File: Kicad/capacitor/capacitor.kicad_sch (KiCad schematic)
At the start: 141 parts, among them K1 Capacitor

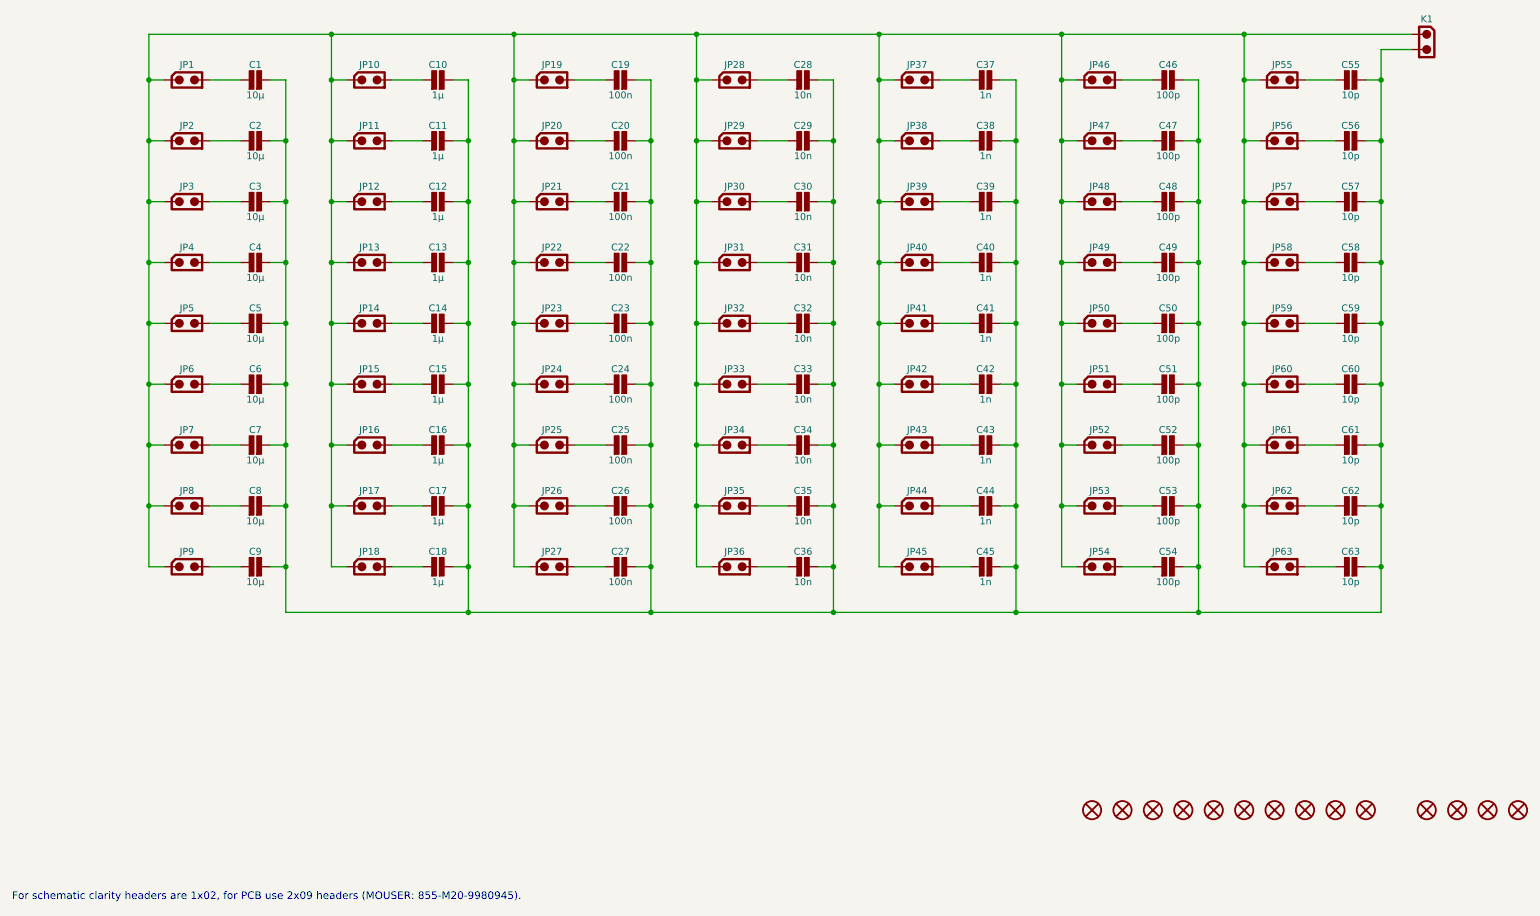
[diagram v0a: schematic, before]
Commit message: Up
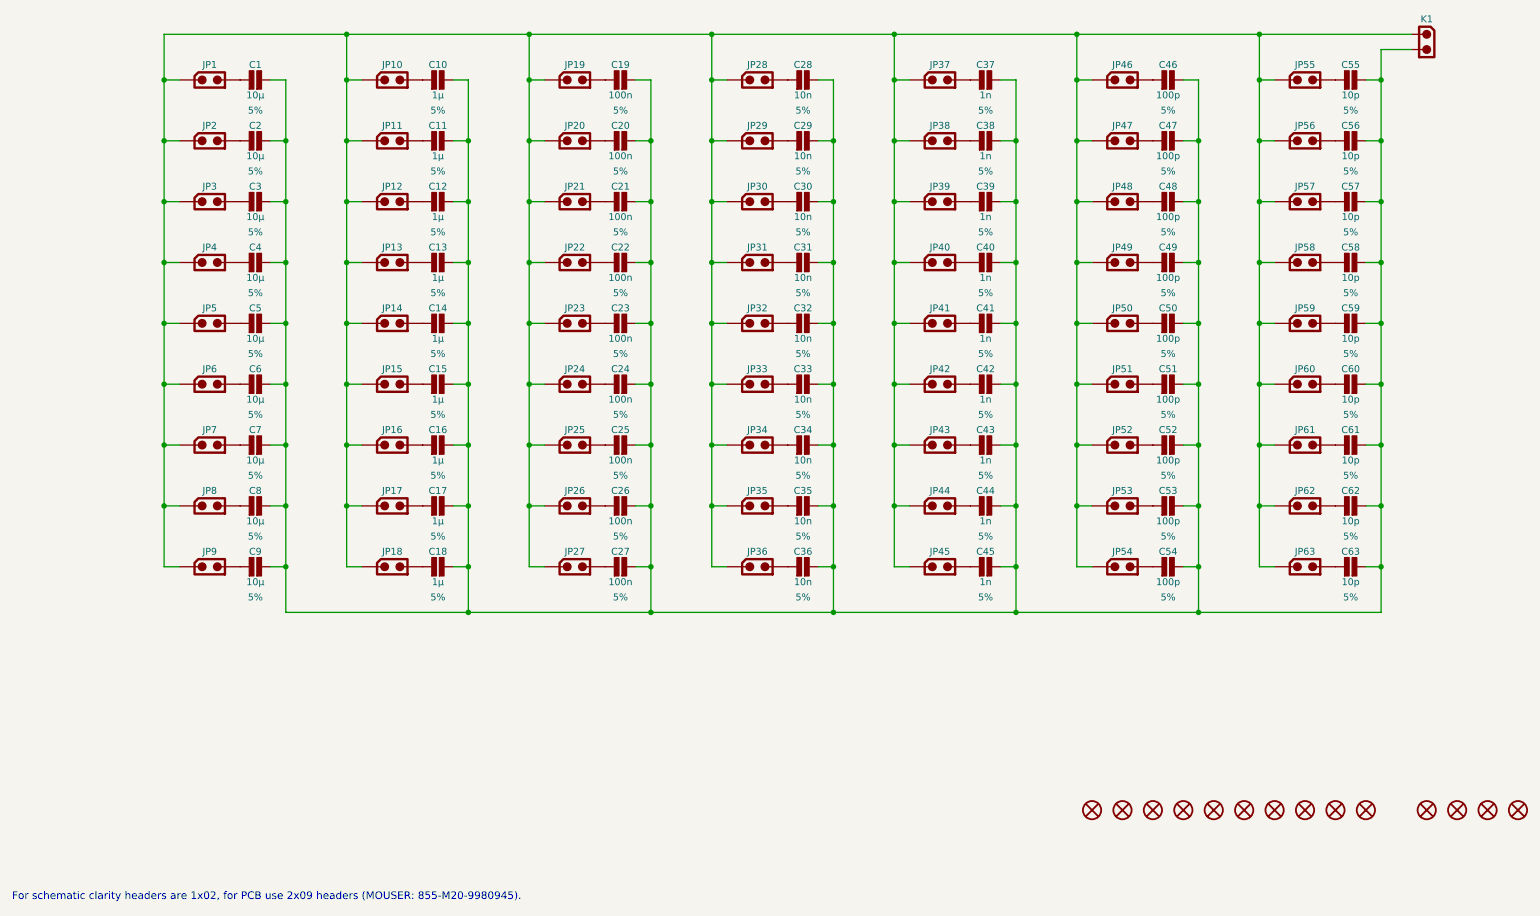
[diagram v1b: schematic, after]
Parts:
- removed C11, C12, C13, C14, C15, C16, C17, C18: 1µ, tronixio:CAPACITOR-SMD-1206, symbol tronixio:CAPACITOR-1206-1U-5P
- removed C2, C3, C4, C5, C6, C7, C8, C9: 10µ, tronixio:CAPACITOR-SMD-1206, symbol tronixio:CAPACITOR-1206-10U-5P
- removed C20, C21, C22, C23, C24, C25, C26, C27: 100n, tronixio:CAPACITOR-SMD-1206, symbol tronixio:CAPACITOR-1206-100N-5P
- removed C29, C30, C31, C32, C33, C34, C35, C36: 10n, tronixio:CAPACITOR-SMD-1206, symbol tronixio:CAPACITOR-1206-10N-5P
- removed C38, C39, C40, C41, C42, C43, C44, C45: 1n, tronixio:CAPACITOR-SMD-1206, symbol tronixio:CAPACITOR-1206-1N-5P
- removed C47, C48, C49, C50, C51, C52, C53, C54: 100p, tronixio:CAPACITOR-SMD-1206, symbol tronixio:CAPACITOR-1206-100P-5P
- removed C56, C57, C58, C59, C60, C61, C62, C63: 10p, tronixio:CAPACITOR-SMD-1206, symbol tronixio:CAPACITOR-1206-10P-5P
- added C11, C12, C13, C14, C15, C16, C17, C18: 1µ, tronixio:CAPACITOR-SMD-1206, symbol tronixio:CAPACITOR-1206-1U-5P-X7R
- added C2, C3, C4, C5, C6, C7, C8, C9: 10µ, tronixio:CAPACITOR-SMD-1206, symbol tronixio:CAPACITOR-1206-10U-5P-X7R
- added C20, C21, C22, C23, C24, C25, C26, C27: 100n, tronixio:CAPACITOR-SMD-1206, symbol tronixio:CAPACITOR-1206-100N-5P-X7R
- added C29, C30, C31, C32, C33, C34, C35, C36: 10n, tronixio:CAPACITOR-SMD-1206, symbol tronixio:CAPACITOR-1206-10N-5P-X7R
- added C38, C39, C40, C41, C42, C43, C44, C45: 1n, tronixio:CAPACITOR-SMD-1206, symbol tronixio:CAPACITOR-1206-1N-5P-COG
- added C47, C48, C49, C50, C51, C52, C53, C54: 100p, tronixio:CAPACITOR-SMD-1206, symbol tronixio:CAPACITOR-1206-100P-5P-COG
- added C56, C57, C58, C59, C60, C61, C62, C63: 10p, tronixio:CAPACITOR-SMD-1206, symbol tronixio:CAPACITOR-1206-10P-5P-COG
- C1: symbol tronixio:CAPACITOR-1206-10U-5P -> tronixio:CAPACITOR-1206-10U-5P-X7R; Name CAPACITOR-1206-10U-5P -> (none); Voltage 50V -> 25V
- C10: symbol tronixio:CAPACITOR-1206-1U-5P -> tronixio:CAPACITOR-1206-1U-5P-X7R; Name CAPACITOR-1206-1U-5P -> (none)
- C19: symbol tronixio:CAPACITOR-1206-100N-5P -> tronixio:CAPACITOR-1206-100N-5P-X7R; Name CAPACITOR-1206-100N-5P -> (none)
- C28: symbol tronixio:CAPACITOR-1206-10N-5P -> tronixio:CAPACITOR-1206-10N-5P-X7R; Name CAPACITOR-1206-10N-5P -> (none)
- C37: symbol tronixio:CAPACITOR-1206-1N-5P -> tronixio:CAPACITOR-1206-1N-5P-COG; Mouser 80-C1206C102J5R -> 80-C1206C103JAGECAUT; Name CAPACITOR-1206-1N-5P -> (none); Voltage 50V -> 250V
- C46: symbol tronixio:CAPACITOR-1206-100P-5P -> tronixio:CAPACITOR-1206-100P-5P-COG; Name CAPACITOR-1206-100P-5P -> (none)
- C55: symbol tronixio:CAPACITOR-1206-10P-5P -> tronixio:CAPACITOR-1206-10P-5P-COG; Name CAPACITOR-1206-10P-5P -> (none)
- JP1, JP10, JP11, JP12, JP13, JP14, JP15, JP16, JP17, JP18, JP19, JP2, JP20, JP21, JP22, JP23, JP24, JP25, JP26, JP27, JP28, JP29, JP3, JP30, JP31, JP32, JP33, JP34, JP35, JP36, JP37, JP38, JP39, JP4, JP40, JP41, JP42, JP43, JP44, JP45, JP46, JP47, JP48, JP49, JP5, JP50, JP51, JP52, JP53, JP54, JP55, JP56, JP57, JP58, JP59, JP6, JP60, JP61, JP62, JP63, JP7, JP8, JP9: Name HARWIN-254-M-1X02-JUMPER-VERTICAL -> (none)
- K1: Name HARWIN-254-M-1X02-VERTICAL -> (none)
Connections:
- net at JP16.2: now also C16.1
- net at C1.2, C10.2, C19.2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: now also C11.2, C12.2, C13.2, C14.2, C15.2, C16.2, C17.2, C18.2, C2.2, C20.2, C21.2, C22.2, C23.2, C24.2, C25.2, C26.2, C27.2, C29.2, C3.2, C30.2, C31.2, C32.2, C33.2, C34.2, C35.2, C36.2, C38.2, C39.2, C4.2, C40.2, C41.2, C42.2, C43.2, C44.2, C45.2, C47.2, C48.2, C49.2, C5.2, C50.2, C51.2, C52.2, C53.2, C54.2, C56.2, C57.2, C58.2, C59.2, C6.2, C60.2, C61.2, C62.2, C63.2, C7.2, C8.2, C9.2
- net at JP61.2: now also C61.1
- net at JP40.2: now also C40.1
- net at JP5.2: now also C5.1
- net at JP22.2: now also C22.1
- net at JP62.2: now also C62.1
- net at JP25.2: now also C25.1
- net at JP35.2: now also C35.1
- net at JP52.2: now also C52.1
- net at JP31.2: now also C31.1
- net at JP33.2: now also C33.1
- net at JP56.2: now also C56.1
- net at JP43.2: now also C43.1
- net at JP18.2: now also C18.1
- net at JP12.2: now also C12.1
- net at JP54.2: now also C54.1
- net at JP44.2: now also C44.1
- net at JP42.2: now also C42.1
- net at JP30.2: now also C30.1
- net at JP38.2: now also C38.1
- net at JP34.2: now also C34.1
- net at JP59.2: now also C59.1
- net at JP6.2: now also C6.1
- net at JP23.2: now also C23.1
- net at JP20.2: now also C20.1
- net at JP32.2: now also C32.1
- net at JP9.2: now also C9.1
- net at JP45.2: now also C45.1
- net at JP14.2: now also C14.1
- net at JP27.2: now also C27.1
- net at JP24.2: now also C24.1
- net at JP21.2: now also C21.1
- net at JP17.2: now also C17.1
- net at JP4.2: now also C4.1
- net at JP15.2: now also C15.1
- net at JP13.2: now also C13.1
- net at JP51.2: now also C51.1
- net at JP53.2: now also C53.1
- net at JP47.2: now also C47.1
- net at JP36.2: now also C36.1
- net at JP48.2: now also C48.1
- net at JP29.2: now also C29.1
- net at JP11.2: now also C11.1
- net at JP2.2: now also C2.1
- net at JP41.2: now also C41.1
- net at JP7.2: now also C7.1
- net at JP3.2: now also C3.1
- net at JP57.2: now also C57.1
- net at JP60.2: now also C60.1
- net at JP58.2: now also C58.1
- net at JP39.2: now also C39.1
- net at JP8.2: now also C8.1
- net at JP49.2: now also C49.1
- net at JP63.2: now also C63.1
- net at JP26.2: now also C26.1
- net at JP50.2: now also C50.1
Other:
- moved on the sheet: JP1
